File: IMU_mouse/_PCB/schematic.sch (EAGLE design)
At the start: 30 parts, among them IC1 REG1117, U1 GY-521MPU6050

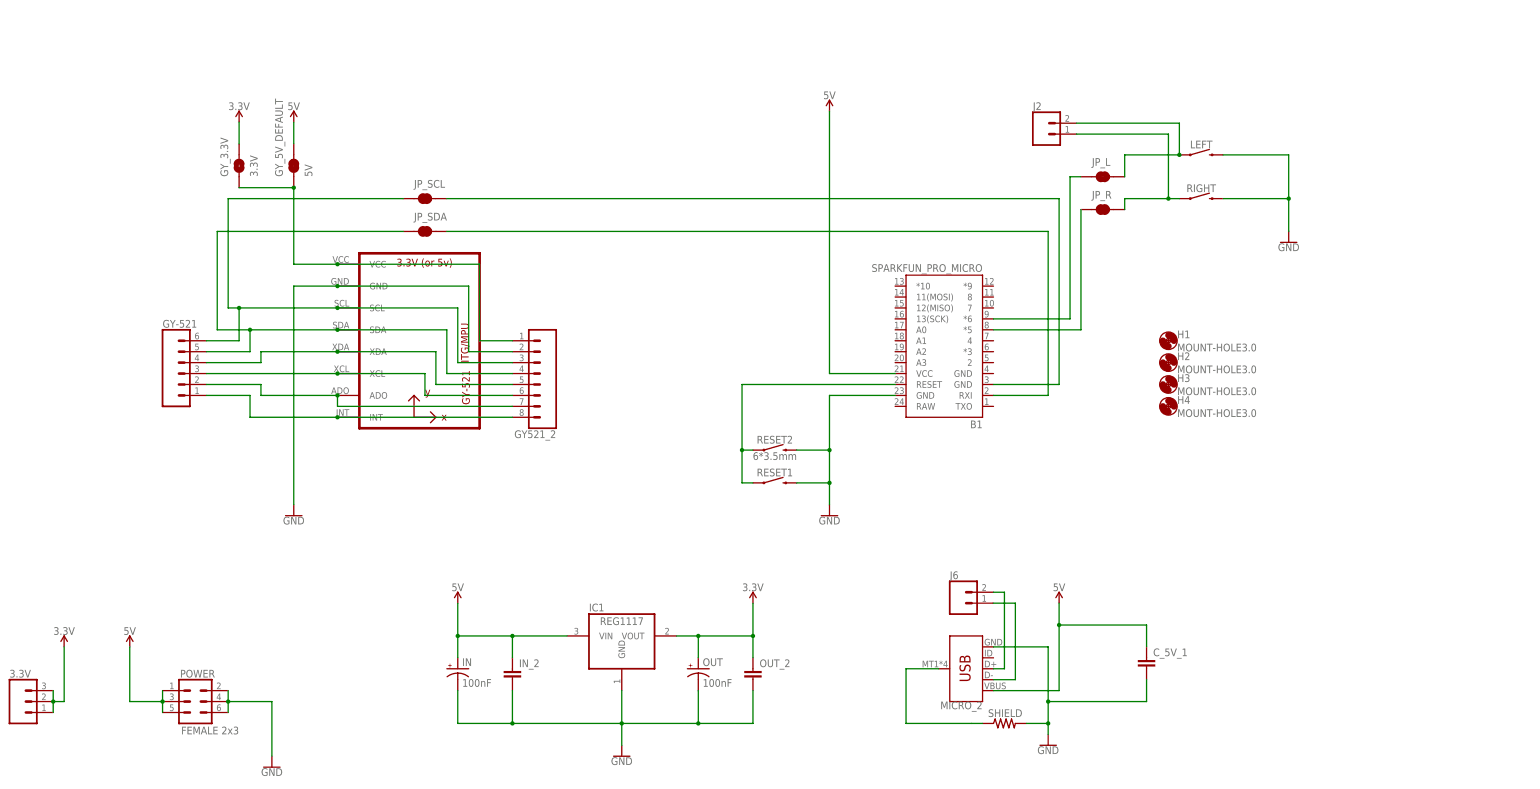
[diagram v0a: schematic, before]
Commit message: IMU mouse update
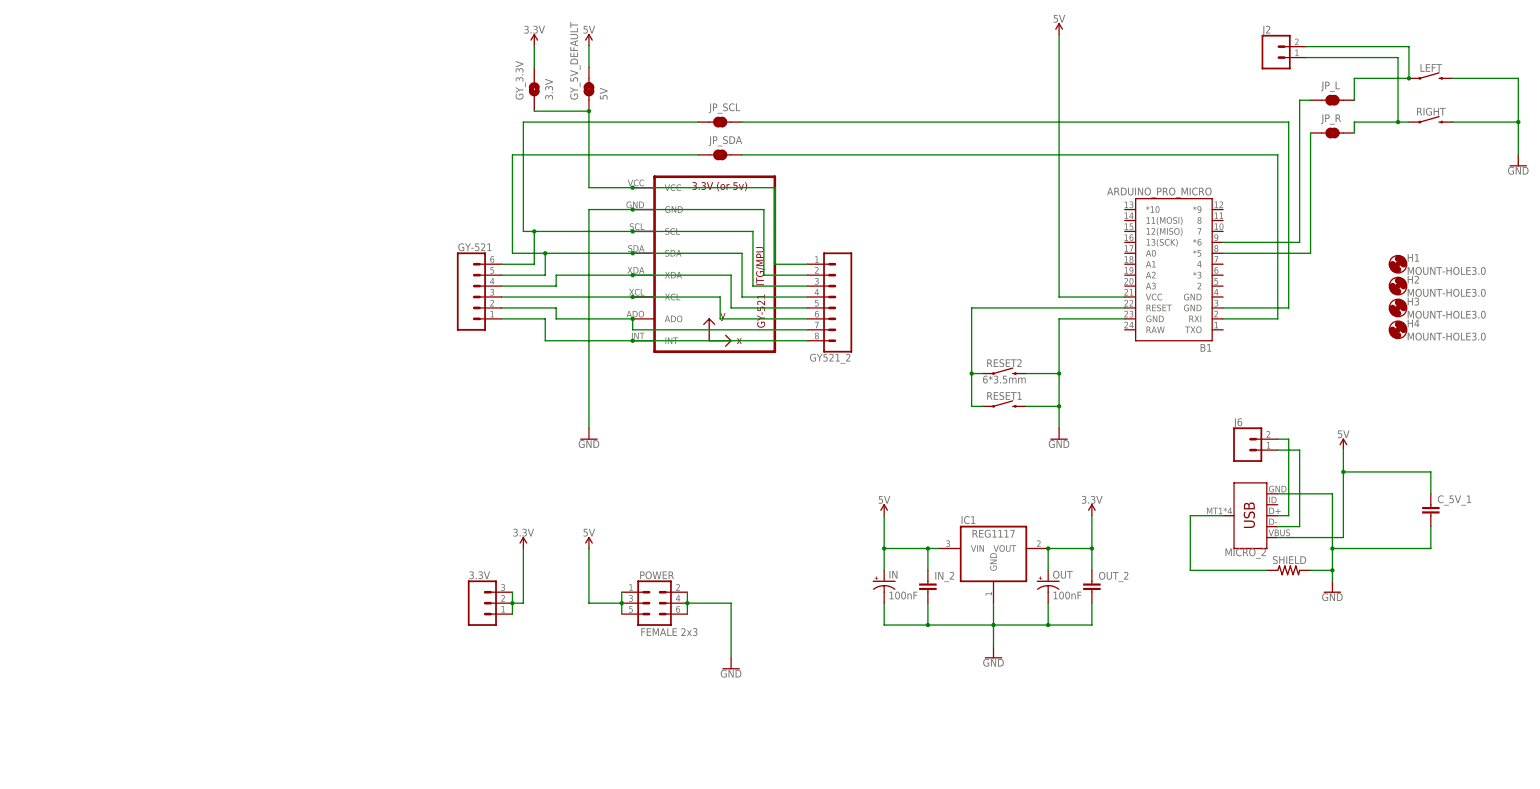
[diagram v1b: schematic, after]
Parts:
- B1: value SPARKFUN_PRO_MICRO -> ARDUINO_PRO_MICRO
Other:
- moved on the sheet: 3.3V, B1, C_5V_1, GY-521, GY521_2, GY_3.3V, GY_5V_DEFAULT, H1, H2, H3, H4, IC1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
